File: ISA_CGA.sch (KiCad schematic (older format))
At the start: 31 parts, among them U1 74S112, U11 74LS74, U12 74LS393, U13 74LS08, U14 74LS32, U15 74LS00, U16 74LS04, U2 74LS74, U20 74LS04, U22 74LS51, U23 74LS32, U25 74LS00, U26 74LS04, U27 74LS51, U28 74LS10, U29 74S04, U3 74S86, U30 74LS32, U31 74S08, U41 74LS08, U42 74LS86, U43 74S74, U44 74S74, U46 74LS00, U47 74LS51, U48 74LS51, U49 74LS02, U6 74LS04, U62 74LS125, U65 74LS02, U68 74LS86

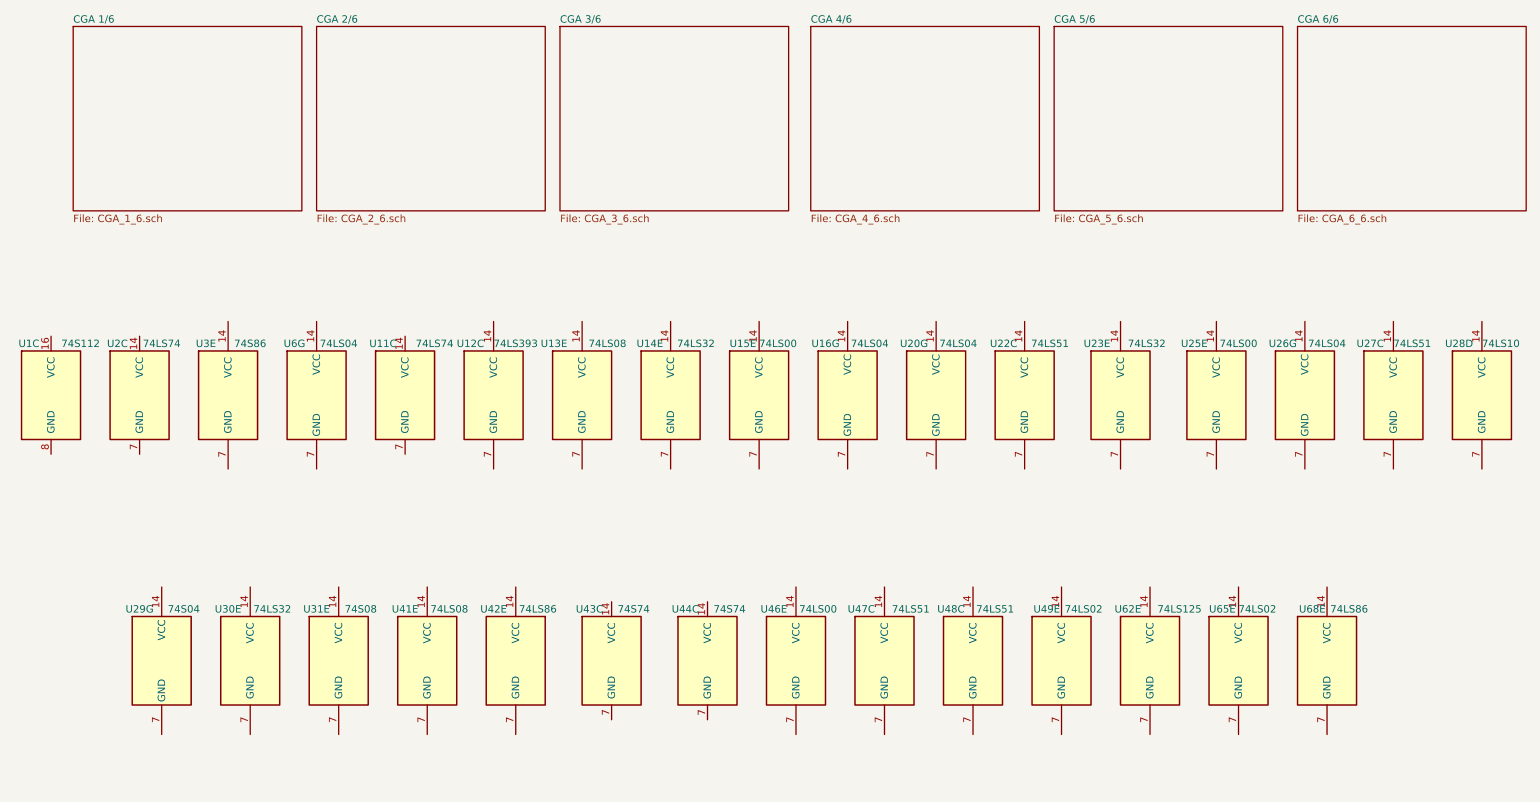
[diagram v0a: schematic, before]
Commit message: Sheet 6
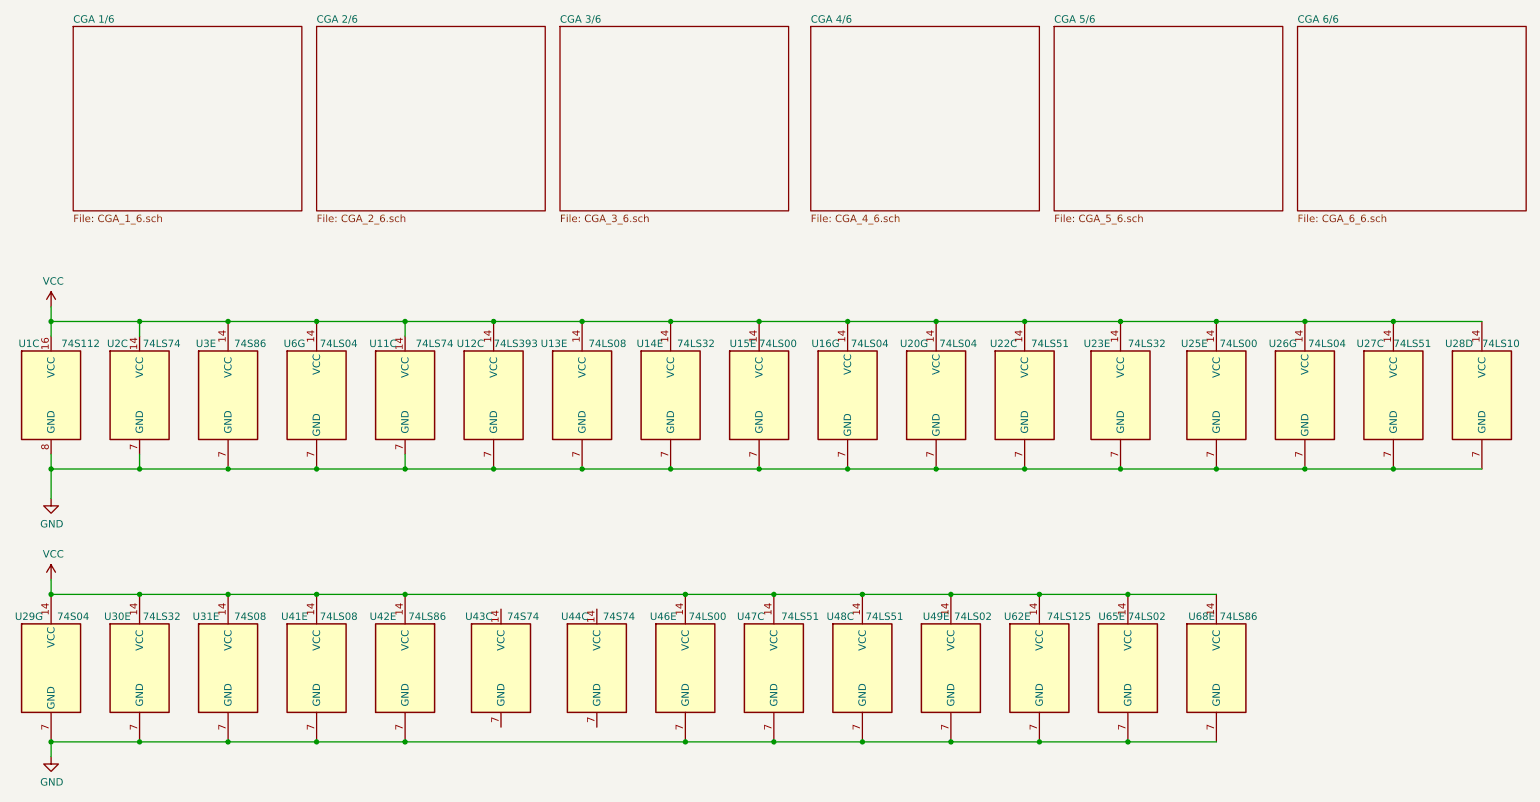
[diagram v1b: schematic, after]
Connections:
- net VCC: now reaches U48.14 (VCC)
- net VCC: now also U1.16 (VCC), U11.14 (VCC), U12.14 (VCC), U13.14 (VCC), U14.14 (VCC), U15.14 (VCC), U16.14 (VCC), U2.14 (VCC), U20.14 (VCC), U22.14 (VCC), U23.14 (VCC), U25.14 (VCC), U26.14 (VCC), U27.14 (VCC), U28.14 (VCC), U29.14 (VCC), U3.14 (VCC), U30.14 (VCC), U31.14 (VCC), U41.14 (VCC), U42.14 (VCC), U46.14 (VCC), U47.14 (VCC), U49.14 (VCC), U6.14 (VCC), U62.14 (VCC), U65.14 (VCC), U68.14 (VCC)
- net GND: now reaches U48.7 (GND)
- net GND: now also U1.8 (GND), U11.7 (GND), U12.7 (GND), U13.7 (GND), U14.7 (GND), U15.7 (GND), U16.7 (GND), U2.7 (GND), U20.7 (GND), U22.7 (GND), U23.7 (GND), U25.7 (GND), U26.7 (GND), U27.7 (GND), U28.7 (GND), U29.7 (GND), U3.7 (GND), U30.7 (GND), U31.7 (GND), U41.7 (GND), U42.7 (GND), U46.7 (GND), U47.7 (GND), U49.7 (GND), U6.7 (GND), U62.7 (GND), U65.7 (GND), U68.7 (GND)
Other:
- moved on the sheet: U29G, U30E, U31E, U41E, U42E, U43C, U44C, U46E, U47C, U48C, U49E, U62E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
